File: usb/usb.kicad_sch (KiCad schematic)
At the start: 23 parts, among them SW1 HX-3X6X2.5-X SMD TACT SWITCH, SW2 HX-3X6X2.5-X SMD TACT SWITCH, U1 SN74LVC125APWR, U2 10kΩ, U3 AMS1117, U4 CH340C, U5 10kΩ, U6 10kΩ, U7 10kΩ, U8 10kΩ, U9 10kΩ

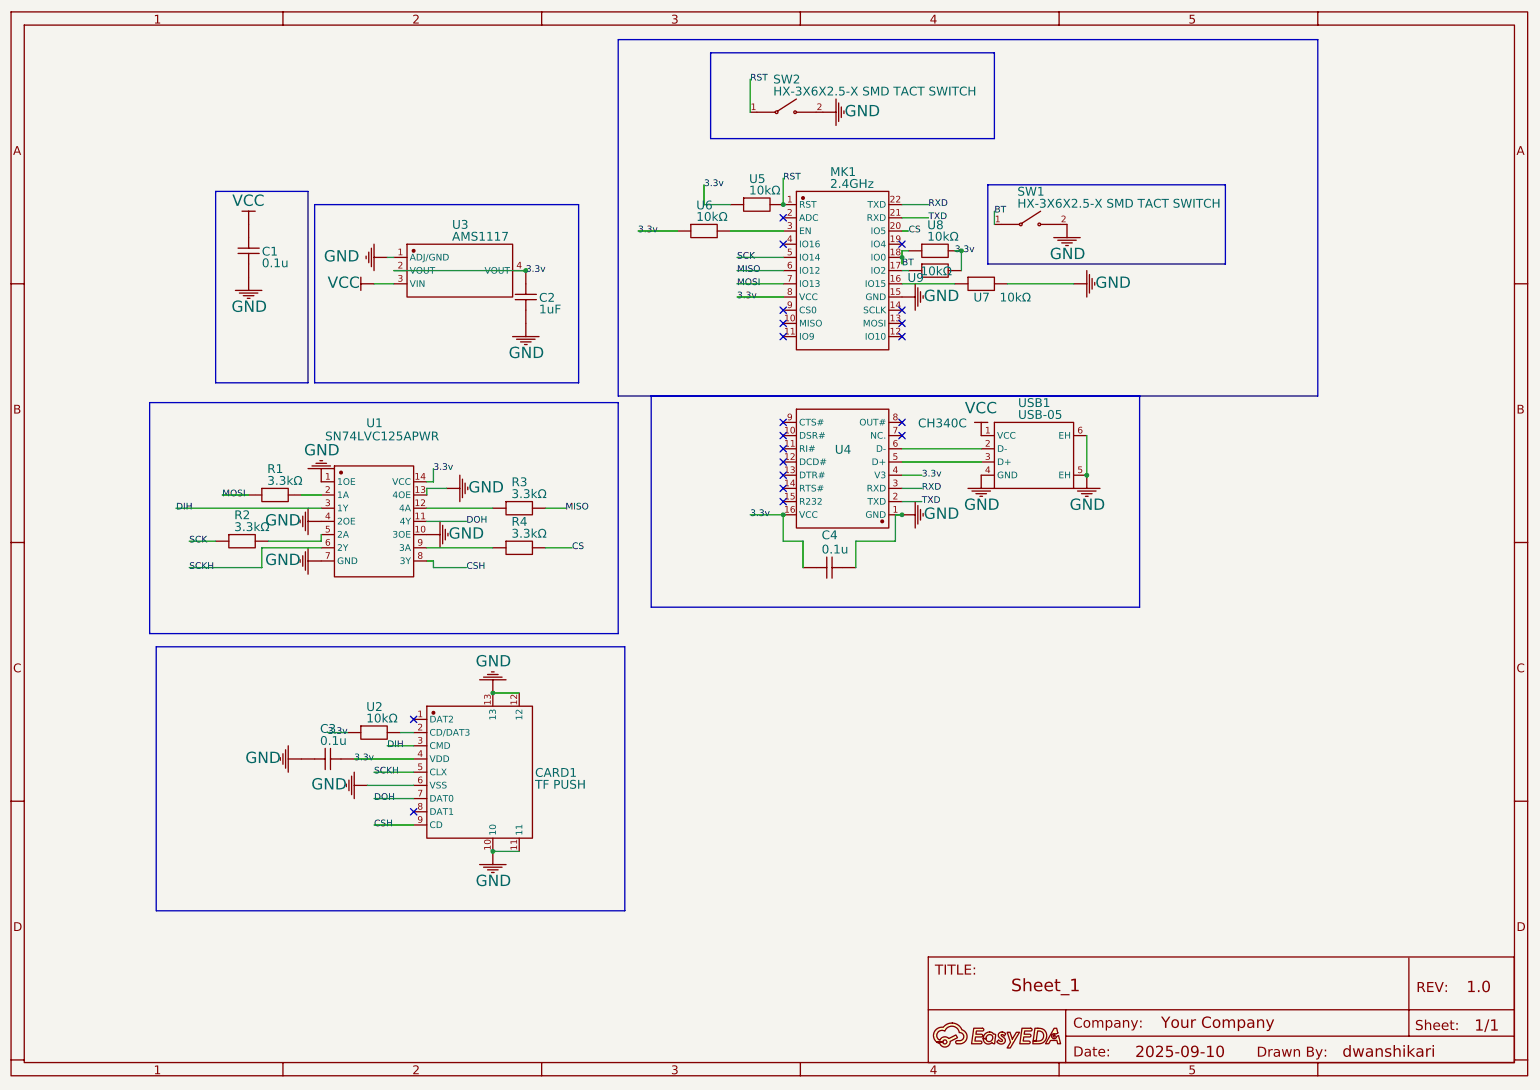
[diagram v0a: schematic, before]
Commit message: kicad
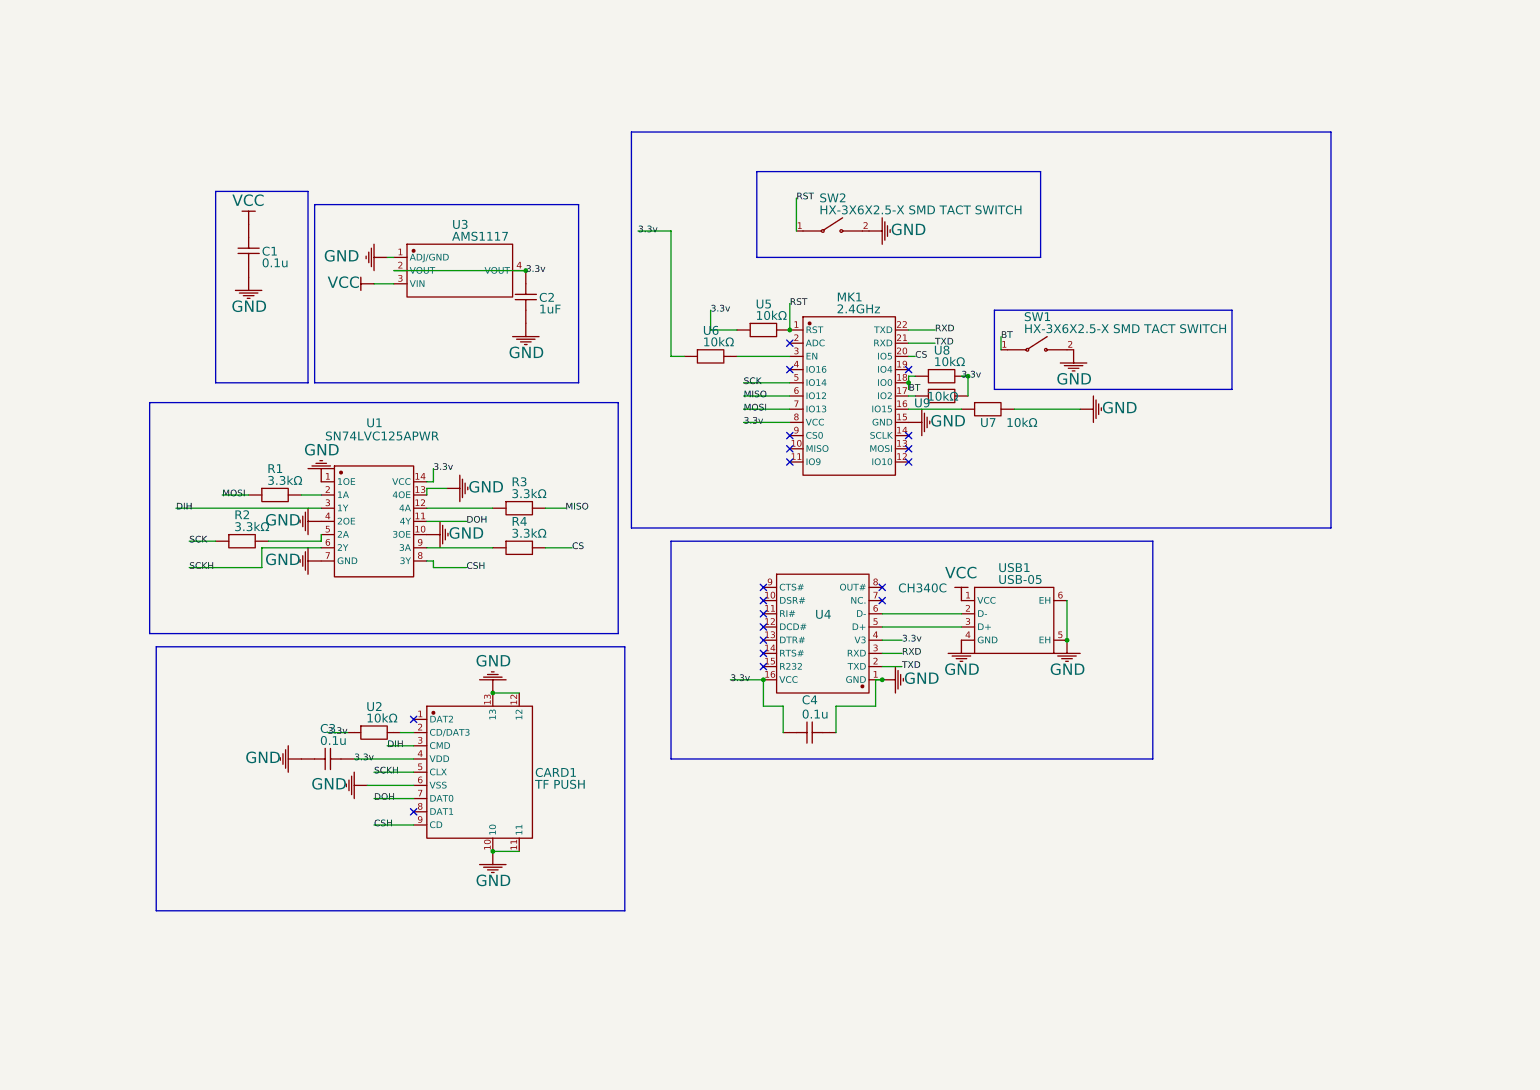
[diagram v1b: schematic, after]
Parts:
- removed A: A, symbol Unknown_0_-806
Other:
- title: (none) -> USB STICK SERVER
- moved on the sheet: C4, MK1, SW1, SW2, U4, U5, U6, U7, U8, U9, USB1
